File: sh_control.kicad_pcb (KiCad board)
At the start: 4 copper layers, 70 x 70 mm, 121 parts, among them IC1 SN65220DBVT, IC2 TUSB2046IBVF, IC3 ATMEGA328P-AU, IC4 FT232RL-REEL, IC5 LM317MDCY, J1 12401598E4#2A, J2 10129381-906001BLF, J3 10129381-906001BLF, Y1 6Mhz, Y2 16 MHz

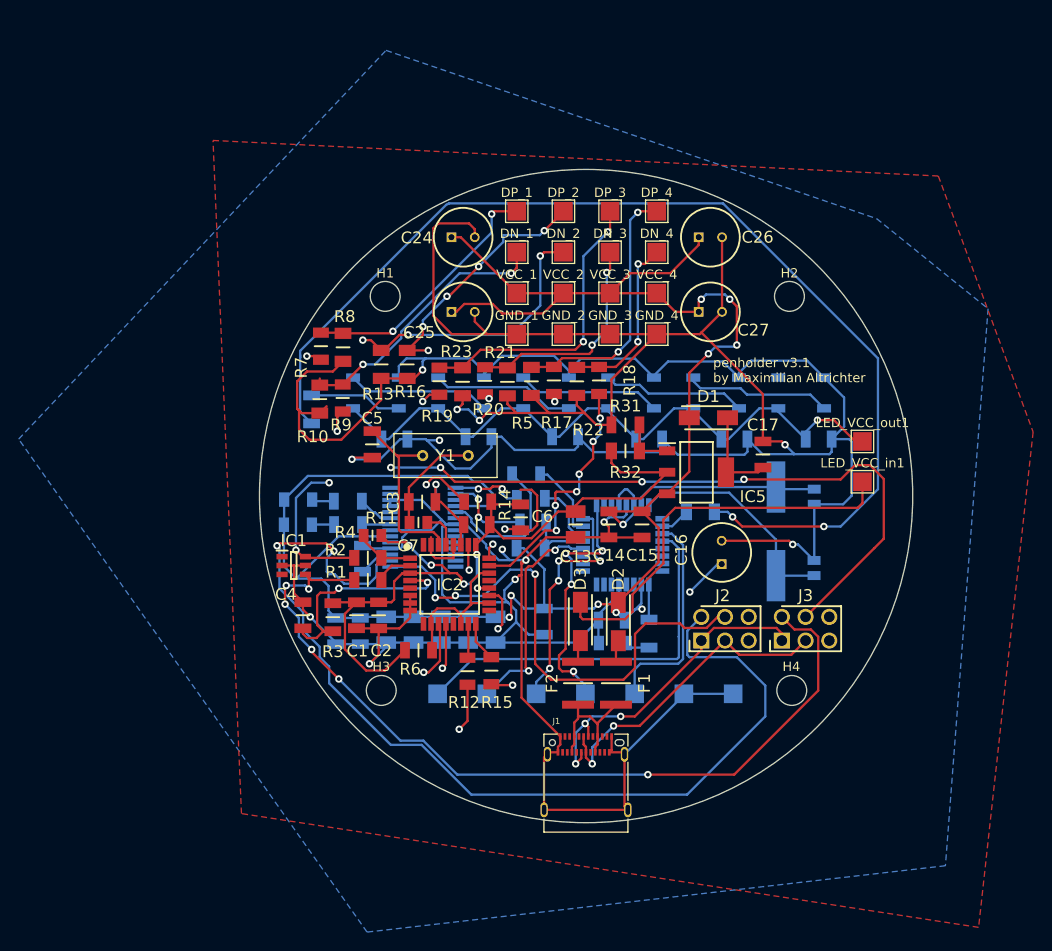
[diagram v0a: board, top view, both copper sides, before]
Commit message: deleted all, beginning of eval board
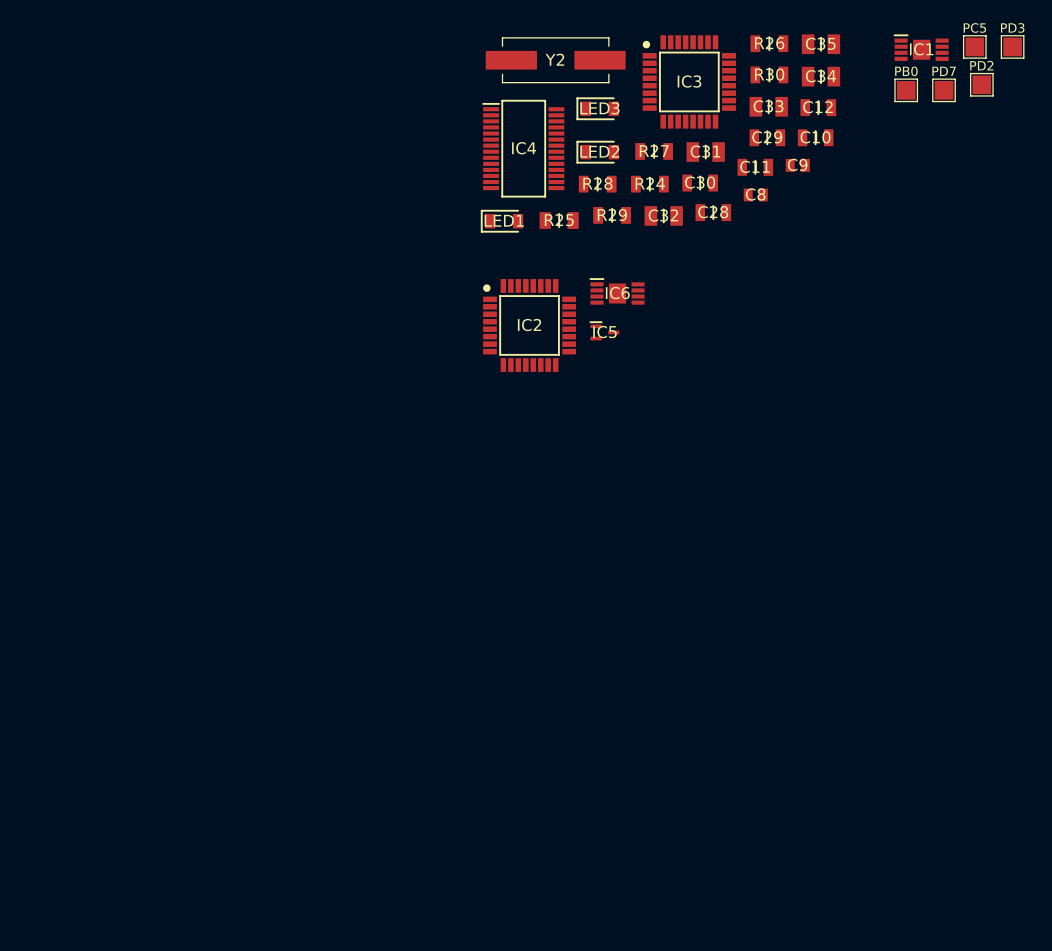
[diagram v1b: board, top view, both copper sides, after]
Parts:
- removed C1, C14, C18, C19, C20, C21, C22, C23, C6: 10 uF, SamacSys_Parts:CAPC3216X180N
- removed C13: 1 uF, SamacSys_Parts:CAPC3216X210N
- removed C15, C17, C2, C4, C7: 0.1 uF, SamacSys_Parts:CAPC3216X88N
- removed C16, C24, C25, C26, C27: 100 uF, SamacSys_Parts:CAPPRD250W45D630H500
- removed C3, C5: 27 pF, SamacSys_Parts:CAPC3216X170N
- removed D1, D2, D3: FM4002-W, SamacSys_Parts:DIOM5025X231N
- removed DN_1, DN_2, DN_3, DN_4, DP_1, DP_2, DP_3, DP_4, GND1, GND2, GND_1, GND_2, GND_3, GND_4, LED_VCC_in1, LED_VCC_out1, VCC_1, VCC_2, VCC_3, VCC_4: TestPoint, TestPoint:TestPoint_Pad_2.0x2.0mm
- removed F1, F2: Fuse, SamacSys_Parts:FUSC4632X85N
- removed H1, H2, H3, H4: MountingHole, MountingHole:MountingHole_3.2mm_M3
- removed J1: 12401598E4#2A, usb c connector:AMPHENOL_12401598E4#2A
- removed J2, J3: 10129381-906001BLF, SamacSys_Parts:HDRV6W67P254_2X3_762X483X858P
- removed LED4, LED5, LED6, LED7, LED8, LED9: COM-13667, SamacSys_Parts:COM13667
- removed R1, R12, R15, R17, R18, R19, R2, R20, R7, R9: 22, SamacSys_Parts:RESC3116X70N
- removed R10, R13, R16, R21, R22, R23, R5, R8: 15K, SamacSys_Parts:RESC3216X75N
- removed R11, R4: 1K5, SamacSys_Parts:RESC2012X60N
- removed R14, R6: 4K7, SamacSys_Parts:RESC3116X65N
- removed R3: 10K, SamacSys_Parts:RESC3216X60N
- removed R31, R33: 390 R, SamacSys_Parts:RESC3216X60N
- removed R32: 240 R, SamacSys_Parts:RESC3216X75N
- removed Y1: 6Mhz, SamacSys_Parts:LFXTAL036567BULK
- added IC6: TLV76733DGNR, SamacSys_Parts:SOP65P490X110-9N, F.Cu at (90.3, 85.0)
- C10, C11, C12, C28, C29, C30, C31, C32, C33, C34, C35, C8, C9, IC3, IC4, LED1, LED2, LED3, PB0, PC5, PD2, PD3, PD7, R24, R25, R26, R27, R28, R29, R30, Y2: moved to F.Cu
- IC1: value SN65220DBVT -> TLV76733DGNR; footprint SamacSys_Parts:SOT95P280X145-6N -> SamacSys_Parts:SOP65P490X110-9N
- IC5: value LM317MDCY -> TPD2E2U06DCKR; footprint SamacSys_Parts:SOT230P700X180-4N -> SamacSys_Parts:SOT65P210X110-3N
- moved IC1 87.1 mm to (122.9, 58.9)
- moved PC5 86.8 mm to (128.6, 58.6)
- moved PD3 83.1 mm to (132.7, 58.6)
- moved PB0 81.9 mm to (121.3, 63.2)
- moved PD2 80.9 mm to (129.4, 62.6)
- moved PD7 72.7 mm to (125.3, 63.2)
- moved C35 71.8 mm to (112.1, 58.3), turned to 0 degrees
- moved C34 70.3 mm to (112.1, 61.7), turned to 0 degrees
- moved C29 70.2 mm to (106.4, 68.3), turned to 0 degrees
- moved C33 66.1 mm to (106.5, 65.0), turned to 0 degrees
- moved R30 66.0 mm to (106.6, 61.6), turned to 0 degrees
- moved C31 61.6 mm to (99.8, 69.8), turned to 0 degrees
- moved C30 60.3 mm to (99.2, 73.1), turned to 0 degrees
- moved C10 59.4 mm to (111.6, 68.3), turned to 0 degrees
- moved C12 59.2 mm to (111.9, 65.1)
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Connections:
- C10 pad 2: USB_GND -> GND
- C12 pad 1: USB_GND -> GND
- C28 pad 2: USB_GND -> GND
- C29 pad 2: USB_GND -> GND
- C30 pad 2: USB_GND -> GND
- C31 pad 2: USB_GND -> GND
- C32 pad 2: USB_GND -> GND
- C33 pad 2: USB_GND -> GND
- C34 pad 2: USB_GND -> GND
- C35 pad 2: USB_GND -> GND
- C8 pad 1: USB_GND -> GND
- C9 pad 1: USB_GND -> GND
- IC1 pad 2: USB_GND -> Net-(IC1-Pad2)
- IC1 pad 4: DN_hub -> Net-(IC1-Pad4)
- IC1 pad 5: USB_GND -> Net-(IC1-Pad5)
- IC1 pad 6: DP_hub -> Net-(IC1-Pad6)
- IC2 pad 14: Net-(IC2-Pad10) -> Net-(IC2-Pad14)
- IC2 pad 18: Net-(IC2-Pad10) -> Net-(IC2-Pad18)
- IC2 pad 22: Net-(IC2-Pad10) -> Net-(IC2-Pad22)
- IC2 pad 25: +3V3 -> Net-(IC2-Pad25)
- IC2 pad 27: USB_GND -> Net-(IC2-Pad27)
- IC2 pad 28: USB_GND -> Net-(IC2-Pad28)
- IC2 pad 3: +3V3 -> Net-(IC2-Pad3)
- IC2 pad 31: USB_GND -> Net-(IC2-Pad31)
- IC2 pad 6: USB_GND -> Net-(IC2-Pad6)
- IC2 pad 7: USB_GND -> Net-(IC2-Pad7)
- IC2 pad 8: USB_GND -> Net-(IC2-Pad8)
- IC3 pad 21: USB_GND -> GND
- IC3 pad 3: USB_GND -> GND
- IC3 pad 5: USB_GND -> GND
- IC4 pad 18: USB_GND -> GND
- IC4 pad 21: USB_GND -> GND
- IC4 pad 25: USB_GND -> GND
- IC4 pad 26: USB_GND -> GND
- IC4 pad 7: USB_GND -> GND
- IC5 pad 2: +3V3 -> Net-(IC5-Pad2)
- IC5 pad 3: VCC -> GND
- LED1 pad 1: USB_GND -> GND
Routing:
- net USB_GND: track 554.8 -> 0.00 mm, vias 15 -> 0
- net VCC: track 233.7 -> 0.00 mm, vias 11 -> 0
- net LED_control: track 117.9 -> 0.00 mm, vias 2 -> 0
- net DN_FT232RL: track 108.1 -> 0.00 mm, vias 2 -> 0
- net DP_hub: track 96.8 -> 0.00 mm, vias 6 -> 0
- net DN_hub: track 92.1 -> 0.00 mm, vias 6 -> 0
- net +3V3: track 86.1 -> 0.00 mm, vias 4 -> 0
- net DN_2: track 83.3 -> 0.00 mm, vias 4 -> 0
- net Net-(C18-Pad2): track 72.2 -> 0.00 mm, vias 1 -> 0
- net DP_2: track 69.3 -> 0.00 mm, vias 6 -> 0
- net Net-(IC2-Pad19): track 67.2 -> 0.00 mm, vias 2 -> 0
- net DP_FT232RL: track 55.5 -> 0.00 mm, vias 3 -> 0
- net Net-(IC2-Pad11): track 47.0 -> 0.00 mm, vias 2 -> 0
- net Net-(IC2-Pad24): track 44.1 -> 0.00 mm, vias 2 -> 0
- net +5V: track 43.2 -> 0.00 mm
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- removed copper zone on B.Cu, net USB_GND
- removed copper zone on F.Cu, net USB_GND
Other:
- board outline removed
- board text removed: "penholder v3.1 by Maximilian Altrichter"
